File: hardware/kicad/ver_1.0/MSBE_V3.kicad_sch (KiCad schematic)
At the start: 88 parts, among them J1 USB_C_Receptacle_USB2.0_16P, J2 Touch Pads, J3 UART, J4 Prog, J6 High-V, J8 Low-V, J9 Low-V-TH, U1 BMA400, U2 MPR121QR2, U3 NRF5340-QKAA-R, U4 NPM1100-CAAA-R7, U6 MAX98357AEWL_T, Y1 32MHz, Y2 32.768kHz

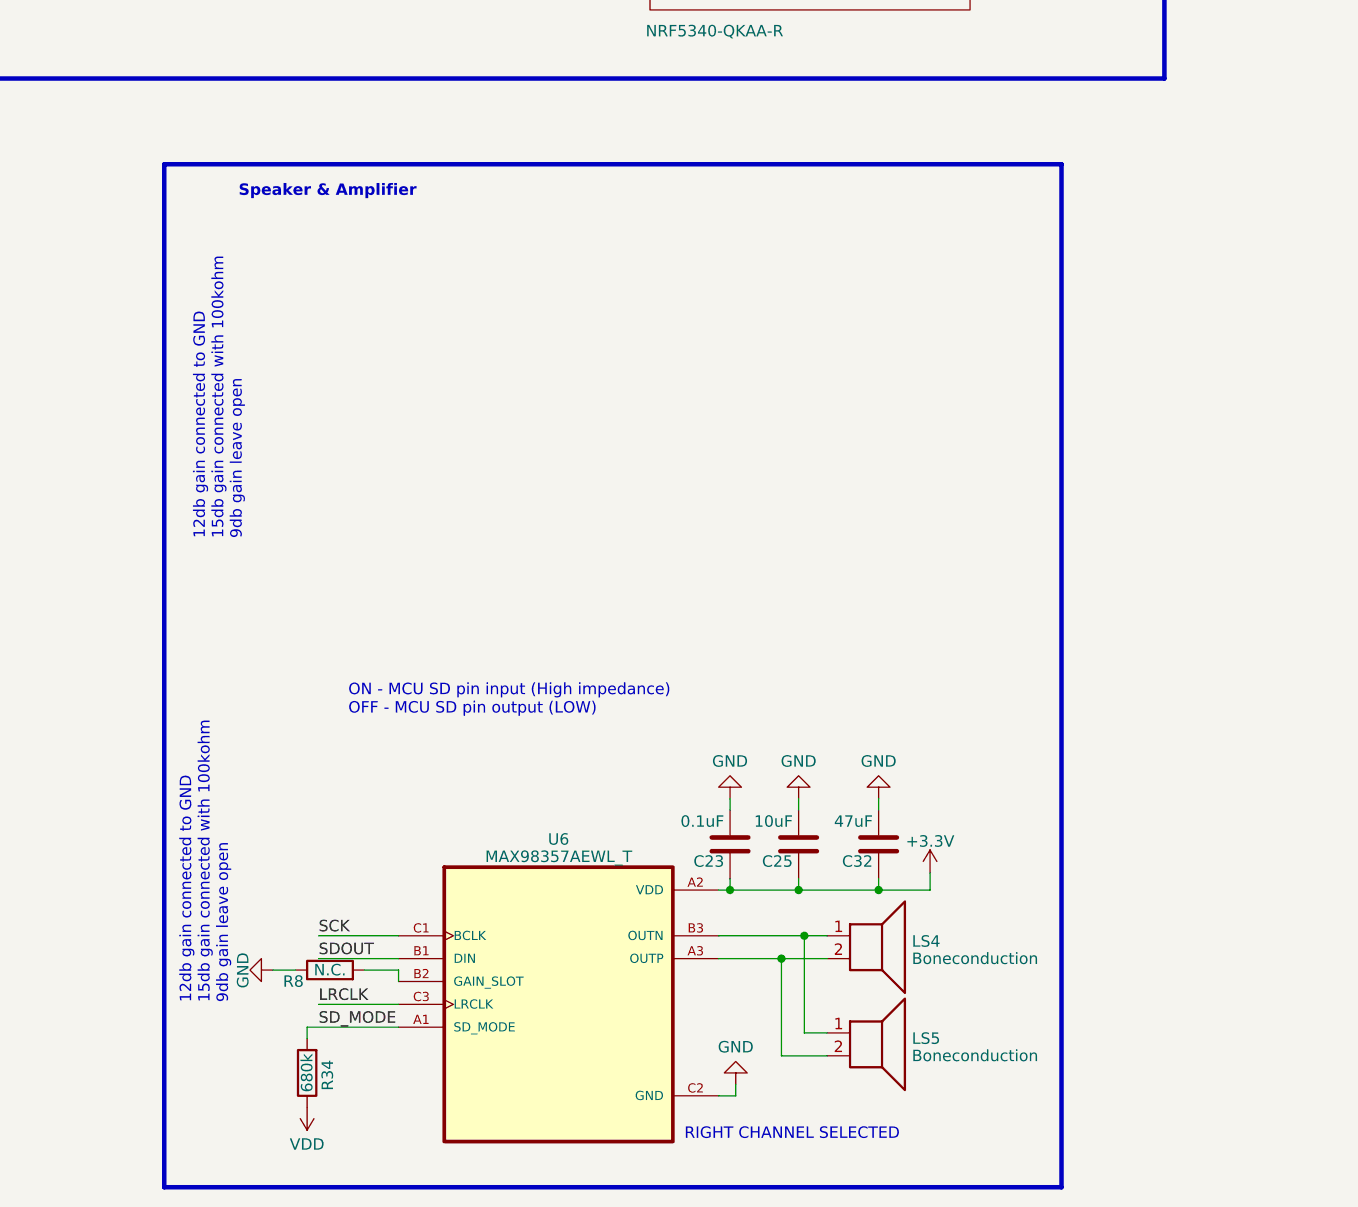
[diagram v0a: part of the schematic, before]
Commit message: newest BGA started
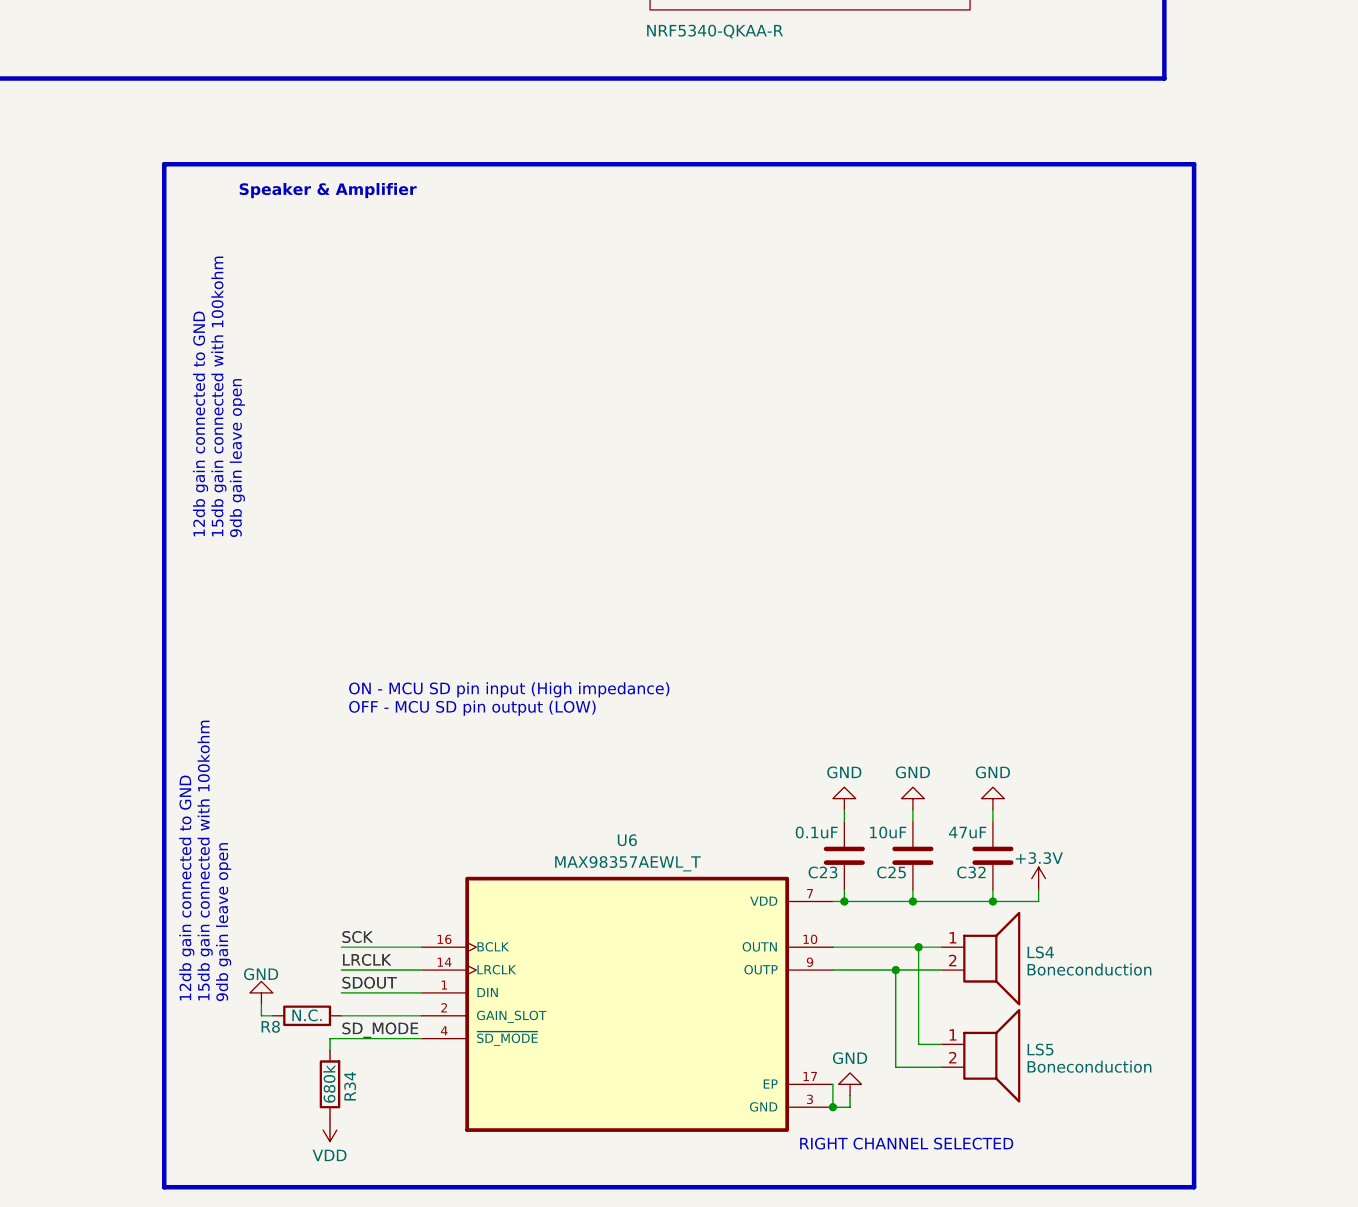
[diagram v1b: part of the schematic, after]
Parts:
- U6: symbol mySch_lib:MAX98357AEWL_T -> lib:MAX98357AETE_
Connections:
- net VDD is gone; now on net +3.3V: C1.1, C10.2, C11.1, C12.1, C15.1, C27.2, C30.1, C31.1, C33.1, C34.1, C35.1, C36.1, C37.1, C38.1, C9.1, J4.1 (Pin_1), L5.1, LS1.5 (VDD), R10.2, R34.1, R9.2, U1.10 (CSB), U1.3 (VDDIO), U1.7 (VDD), U2.20 (VDD), U3.A19 (VDD), U3.AC1 (VDD), U3.AG1 (VDD), U3.AJ31 (VDD), U3.AL11 (VDD), U3.AL17 (VDD), U3.AL25 (VDD), U3.AL3 (VDD), U3.AL7 (VDD), U3.B28 (VDD), U3.B8 (VDD), U3.C1 (VDD), U3.E1 (VDDH), U3.E31 (VDD), U3.L1 (VDD), U3.N31 (VDD), U3.U1 (VDD), U4.B5 (VOUTB), U4.C3 (VTERMSET)
- net +3.3V: now also U6.7 (VDD), U6.8 (VDD); no longer U6.A2 (VDD)
- net AVSS: now also U6.11 (GND), U6.15 (GND), U6.17 (EP), U6.3 (GND); no longer U6.C2 (GND)
- net LRCLK: now also U6.14 (LRCLK); no longer U6.C3 (LRCLK)
- net SCK: now also U6.16 (BCLK); no longer U6.C1 (BCLK)
- net SDOUT: now also U6.1 (DIN); no longer U6.B1 (DIN)
- net SD_MODE: now also U6.4 (~{SD_MODE}); no longer U6.A1 (SD_MODE)
- net at R8.2: now also U6.2 (GAIN_SLOT); no longer U6.B2 (GAIN_SLOT)
- net at LS4.1, LS5.1: now also U6.10 (OUTN); no longer U6.B3 (OUTN)
- net at LS4.2, LS5.2: now also U6.9 (OUTP); no longer U6.A3 (OUTP)
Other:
- moved on the sheet: C23, C25, C32, LS4, LS5, R34, R8
